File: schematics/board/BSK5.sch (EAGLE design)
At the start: 88 parts, among them U1 STM32F405RGT6, X1 JST-6, X11 JST-6

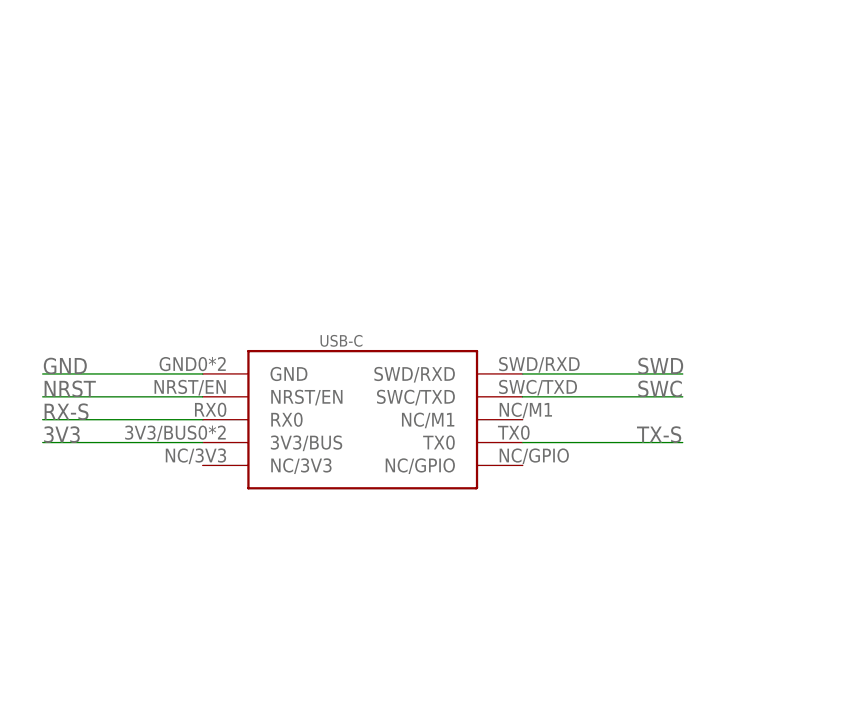
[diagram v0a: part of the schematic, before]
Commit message: Схема БКУ
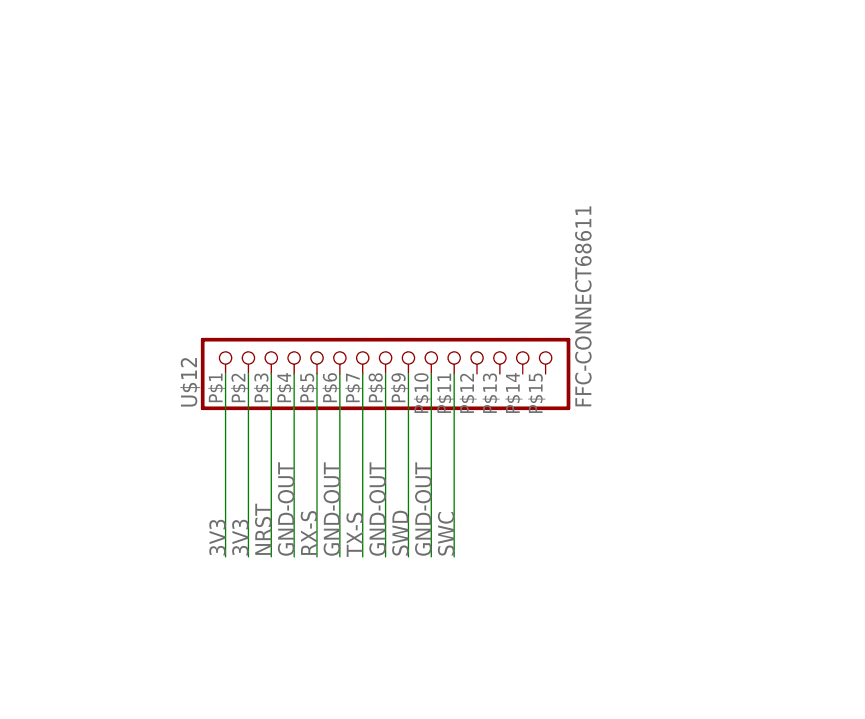
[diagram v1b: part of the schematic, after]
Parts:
- removed U$6: USB-C, CanCubeSat:USB-C
- added U$12: FFC-CONNECT68611, CanCubeSat:FFC-CONNECT68611
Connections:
- net 3V3: now also U$12.1, U$12.2; no longer U$6.3V3/BUS
- net GND: no longer U$6.GND
- net GND-OUT: now also U$12.10, U$12.4, U$12.6, U$12.8
- net NRST: now also U$12.3; no longer U$6.NRST/EN
- net RX-S: now also U$12.5; no longer U$6.RX0
- net SWC: now also U$12.11; no longer U$6.SWC/TXD
- net SWD: now also U$12.9; no longer U$6.SWD/RXD
- net TX-S: now also U$12.7; no longer U$6.TX0
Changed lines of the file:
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@@
 <part name="U1" library="STM32F405RGT6" deviceset="STM32F405RGT6" device=""/>
 <part name="GPS" library="CanCubeSat" deviceset="GPS" device="NEO6M" value="GPSNEO6M"/>
-<part name="U$6" library="CanCubeSat" deviceset="USB-C" device=""/>
 <part name="R1" library="resistor" deviceset="R-US_" device="R0603" package3d_urn="urn:adsk.eagle:package:23555/3" value="10k"/>
 <part name="R15" library="resistor" deviceset="R-US_" device="R0603" package3d_urn="urn:adsk.eagle:package:23555/3" value="2k"/>
@@
 <part name="R31" library="resistor" deviceset="R-US_" device="R0603" package3d_urn="urn:adsk.eagle:package:23555/3" value="100R"/>
 <part name="R32" library="resistor" deviceset="R-US_" device="R0603" package3d_urn="urn:adsk.eagle:package:23555/3" value="100R"/>
+<part name="U$12" library="CanCubeSat" deviceset="FFC-CONNECT" device="68611"/>
 </parts>
 <sheets>
@@
 <attribute name="NAME" x="442.722" y="241.3" size="1.778" layer="95" rot="R270"/>
 </instance>
-<instance part="U$6" gate="G$1" x="88.9" y="264.16" smashed="yes"/>
 <instance part="R1" gate="G$1" x="411.48" y="193.04" smashed="yes" rot="R90">
 <attribute name="NAME" x="409.9814" y="189.23" size="1.778" layer="95" rot="R90"/>
@@
 <attribute name="VALUE" x="519.938" y="306.07" size="1.778" layer="96" rot="R270"/>
 </instance>
+<instance part="U$12" gate="G$1" x="91.44" y="271.78" smashed="yes" rot="R90">
+<attribute name="NAME" x="70.485" y="265.43" size="1.778" layer="95" rot="R90"/>
+<attribute name="VALUE" x="114.3" y="265.43" size="1.778" layer="96" rot="R90"/>
+</instance>
 </instances>
 <busses>
@@
 <nets>
 <net name="GND" class="0">
-<segment>
-<pinref part="U$6" gate="G$1" pin="GND"/>
-<wire x1="71.12" y1="269.24" x2="53.34" y2="269.24" width="0.1524" layer="91"/>
-<label x="53.34" y="269.24" size="1.778" layer="95"/>
-</segment>
 <segment>
 <pinref part="SUPPLY1" gate="GND" pin="GND"/>
@@
 <net name="SWD" class="0">
 <segment>
-<pinref part="U$6" gate="G$1" pin="SWD/RXD"/>
-<wire x1="106.68" y1="269.24" x2="124.46" y2="269.24" width="0.1524" layer="91"/>
-<label x="119.38" y="269.24" size="1.778" layer="95"/>
-</segment>
-<segment>
 <pinref part="U1" gate="G$1" pin="PA13/JMS-SWDIO"/>
 <wire x1="360.68" y1="149.86" x2="421.64" y2="149.86" width="0.1524" layer="91"/>
@@
 <pinref part="R2" gate="G$1" pin="1"/>
 </segment>
+<segment>
+<wire x1="93.98" y1="269.24" x2="93.98" y2="248.92" width="0.1524" layer="91"/>
+<label x="93.98" y="248.92" size="1.778" layer="95" rot="R90"/>
+<pinref part="U$12" gate="G$1" pin="9"/>
+</segment>
 </net>
 <net name="RX-S" class="0">
-<segment>
-<wire x1="53.34" y1="264.16" x2="71.12" y2="264.16" width="0.1524" layer="91"/>
-<label x="53.34" y="264.16" size="1.778" layer="95"/>
-<pinref part="U$6" gate="G$1" pin="RX0"/>
-</segment>
 <segment>
 <pinref part="U1" gate="G$1" pin="PC10"/>
@@
 <label x="487.68" y="157.48" size="1.778" layer="95"/>
 </segment>
+<segment>
+<wire x1="83.82" y1="269.24" x2="83.82" y2="248.92" width="0.1524" layer="91"/>
+<label x="83.82" y="248.92" size="1.778" layer="95" rot="R90"/>
+<pinref part="U$12" gate="G$1" pin="5"/>
+</segment>
 </net>
 <net name="TX-S" class="0">
-<segment>
-<wire x1="124.46" y1="261.62" x2="106.68" y2="261.62" width="0.1524" layer="91"/>
-<label x="119.38" y="261.62" size="1.778" layer="95"/>
-<pinref part="U$6" gate="G$1" pin="TX0"/>
-</segment>
 <segment>
 <pinref part="U1" gate="G$1" pin="PC11"/>
@@
 <label x="487.68" y="154.94" size="1.778" layer="95"/>
 </segment>
+<segment>
+<wire x1="88.9" y1="269.24" x2="88.9" y2="248.92" width="0.1524" layer="91"/>
+<label x="88.9" y="248.92" size="1.778" layer="95" rot="R90"/>
+<pinref part="U$12" gate="G$1" pin="7"/>
+</segment>
 </net>
 <net name="SWC" class="0">
-<segment>
-<wire x1="124.46" y1="266.7" x2="106.68" y2="266.7" width="0.1524" layer="91"/>
-<label x="119.38" y="266.7" size="1.778" layer="95"/>
-<pinref part="U$6" gate="G$1" pin="SWC/TXD"/>
-</segment>
 <segment>
 <pinref part="U1" gate="G$1" pin="PA14/JTCK-SWCLK"/>
@@
 <pinref part="R3" gate="G$1" pin="1"/>
 </segment>
+<segment>
+<wire x1="99.06" y1="269.24" x2="99.06" y2="248.92" width="0.1524" layer="91"/>
+<label x="99.06" y="248.92" size="1.778" layer="95" rot="R90"/>
+<pinref part="U$12" gate="G$1" pin="11"/>
+</segment>
 </net>
 <net name="NRST" class="0">
-<segment>
-<wire x1="53.34" y1="266.7" x2="71.12" y2="266.7" width="0.1524" layer="91"/>
-<label x="53.34" y="266.7" size="1.778" layer="95"/>
-<pinref part="U$6" gate="G$1" pin="NRST/EN"/>
-</segment>
 <segment>
 <pinref part="U1" gate="G$1" pin="NRST"/>
@@
 <junction x="411.48" y="187.96"/>
 <label x="398.78" y="187.96" size="1.778" layer="95"/>
+</segment>
+<segment>
+<pinref part="U$12" gate="G$1" pin="3"/>
+<wire x1="78.74" y1="269.24" x2="78.74" y2="248.92" width="0.1524" layer="91"/>
+<label x="78.74" y="248.92" size="1.778" layer="95" rot="R90"/>
 </segment>
 </net>
@@
 <wire x1="510.54" y1="187.96" x2="482.6" y2="187.96" width="0.1524" layer="91"/>
 <wire x1="482.6" y1="187.96" x2="482.6" y2="195.58" width="0.1524" layer="91"/>
-</segment>
-<segment>
-<wire x1="71.12" y1="261.62" x2="53.34" y2="261.62" width="0.1524" layer="91"/>
-<label x="53.34" y="261.62" size="1.778" layer="95"/>
-<pinref part="U$6" gate="G$1" pin="3V3/BUS"/>
 </segment>
 <segment>
@@
 <label x="551.18" y="121.92" size="1.778" layer="95"/>
 </segment>
+<segment>
+<pinref part="U$12" gate="G$1" pin="2"/>
+<wire x1="76.2" y1="269.24" x2="76.2" y2="248.92" width="0.1524" layer="91"/>
+<label x="76.2" y="248.92" size="1.778" layer="95" rot="R90"/>
+</segment>
+<segment>
+<pinref part="U$12" gate="G$1" pin="1"/>
+<wire x1="73.66" y1="269.24" x2="73.66" y2="248.92" width="0.1524" layer="91"/>
+<label x="73.66" y="248.92" size="1.778" layer="95" rot="R90"/>
+</segment>
 </net>
 <net name="SINS-KVCC" class="0">
@@
 <pinref part="BSK3" gate="A" pin="4"/>
 </segment>
-</net>
+<segment>
+<wire x1="96.52" y1="269.24" x2="96.52" y2="248.92" width="0.1524" layer="91"/>
+<label x="96.52" y="248.92" size="1.778" layer="95" rot="R90"/>
+<pinref part="U$12" gate="G$1" pin="10"/>
+</segment>
+<segment>
+<wire x1="91.44" y1="269.24" x2="91.44" y2="248.92" width="0.1524" layer="91"/>
+<label x="91.44" y="248.92" size="1.778" layer="95" rot="R90"/>
+<pinref part="U$12" gate="G$1" pin="8"/>
+</segment>
+<segment>
+<pinref part="U$12" gate="G$1" pin="6"/>
+<wire x1="86.36" y1="269.24" x2="86.36" y2="248.92" width="0.1524" layer="91"/>
+<label x="86.36" y="248.92" size="1.778" layer="95" rot="R90"/>
+</segment>
+<segment>
+<pinref part="U$12" gate="G$1" pin="4"/>
+<wire x1="81.28" y1="269.24" x2="81.28" y2="248.92" width="0.1524" layer="91"/>
+<label x="81.28" y="248.92" size="1.778" layer="95" rot="R90"/>
+</segment>
+</net>
